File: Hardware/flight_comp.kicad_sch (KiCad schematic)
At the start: 43 parts, among them J2 ARM_SWD_TC2030, J4 USB_C_Receptacle_USB2.0_16P, Q5 PMBT2222A, SW1 NRST, SW2 BOOT0, U1 STM32F405RGTx, U4 W25Q32JVSS, U5 24LC64, U8 USBLC6-2SC6, Y1 8mHz, Y2 32.768 kHz

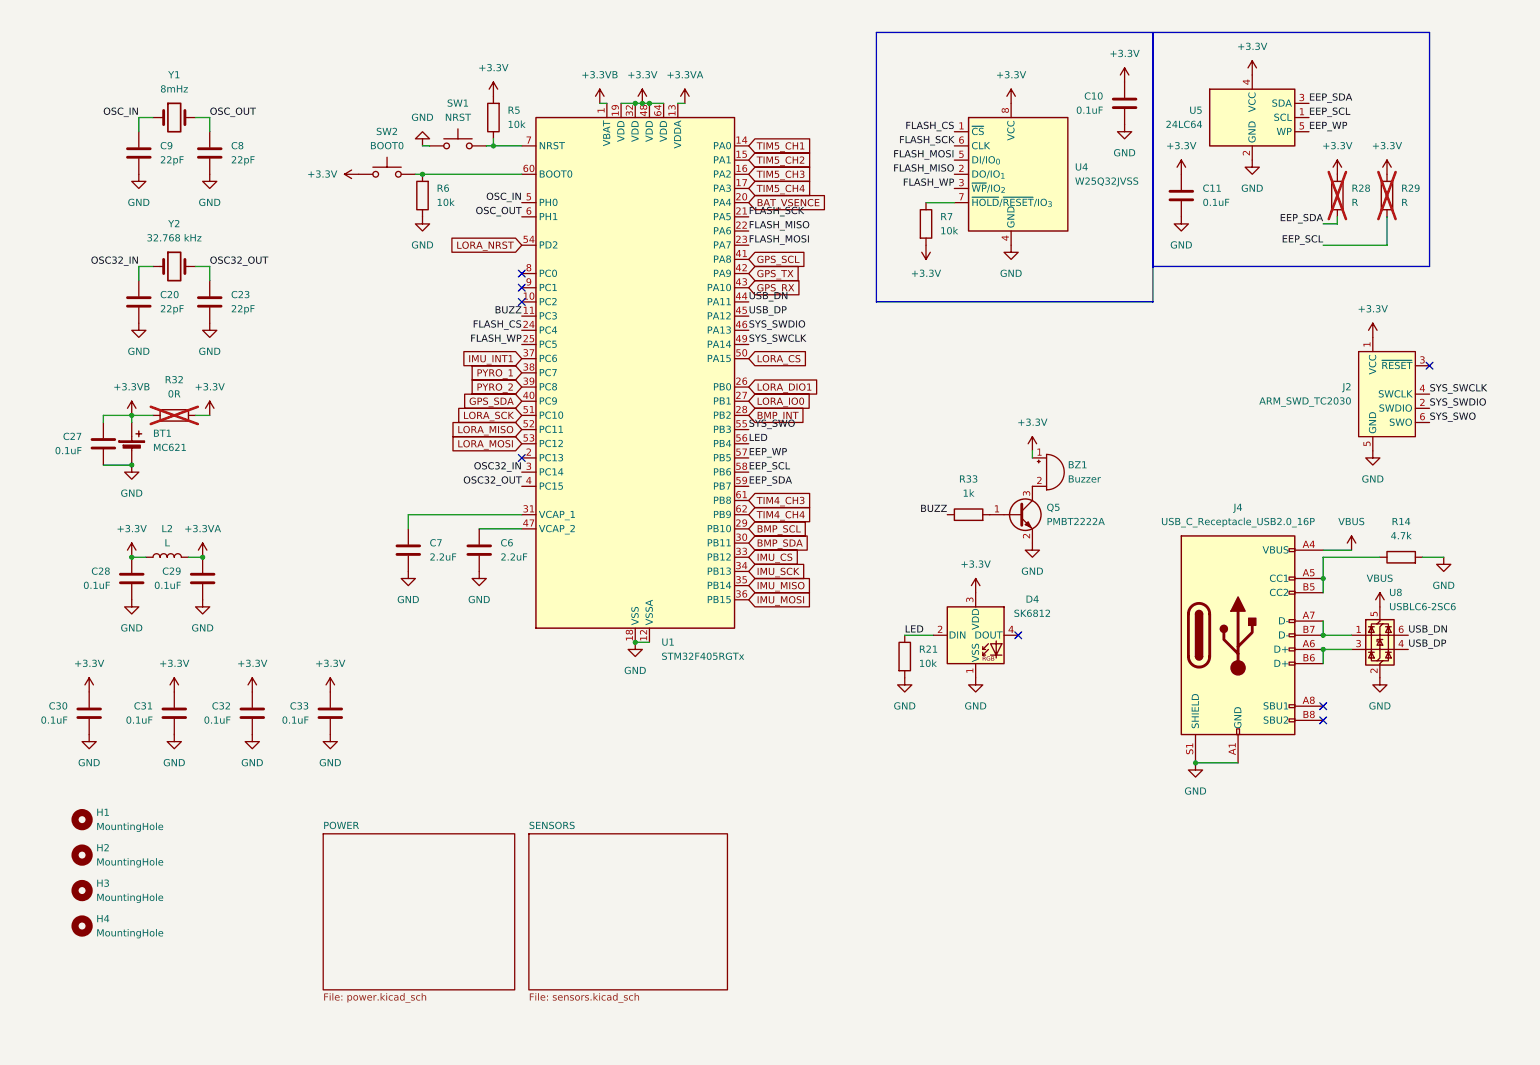
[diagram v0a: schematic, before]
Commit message: Kaut ko palaboju
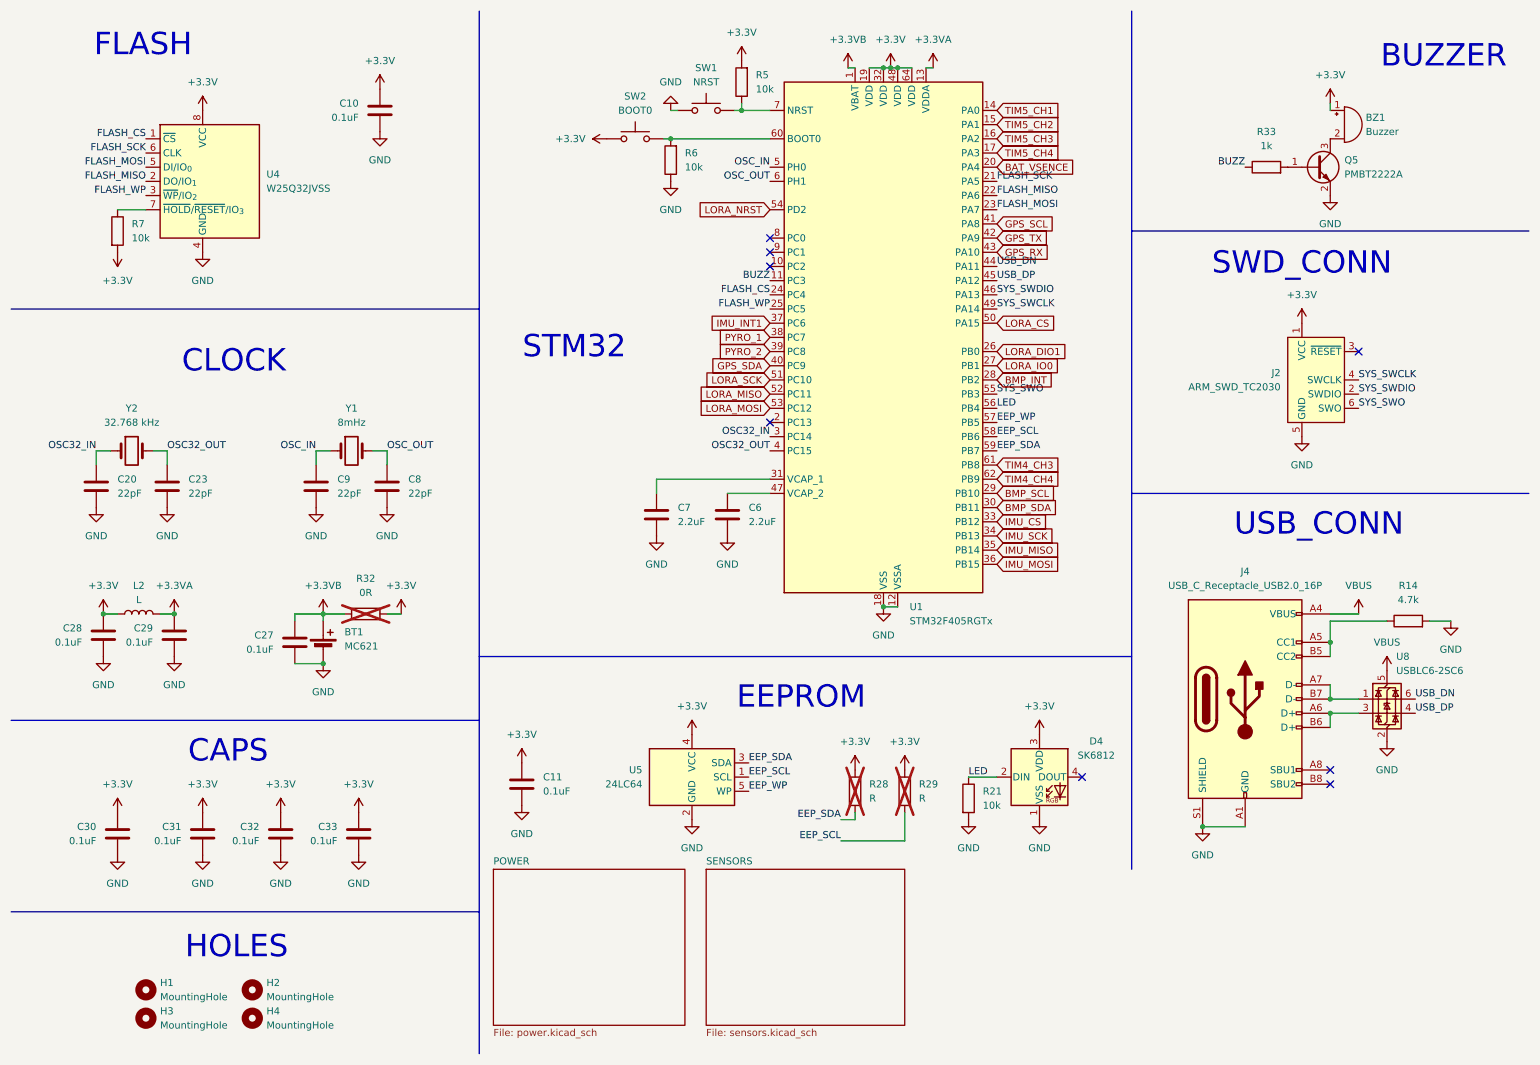
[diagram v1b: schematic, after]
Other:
- note added: "BUZZER"
- note added: "CAPS"
- note added: "CLOCK"
- note added: "EEPROM"
- note added: "FLASH"
- note added: "HOLES"
- note added: "STM32"
- note added: "SWD_CONN"
- note added: "USB_CONN"
- moved on the sheet: BT1, BZ1, C10, C11, C20, C23, C27, C28, C29, C30, C31, C32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
